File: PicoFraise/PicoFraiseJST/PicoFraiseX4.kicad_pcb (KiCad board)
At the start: 2 copper layers, 112.8 x 110 mm, 76 parts, among them J1 Conn_01x06, J2 Conn_01x06, J3 Conn_01x06, J4 Conn_01x06, J5 Conn_01x09, J7 Reset, J8 12-24V input, U1 Pico, U2 L7805

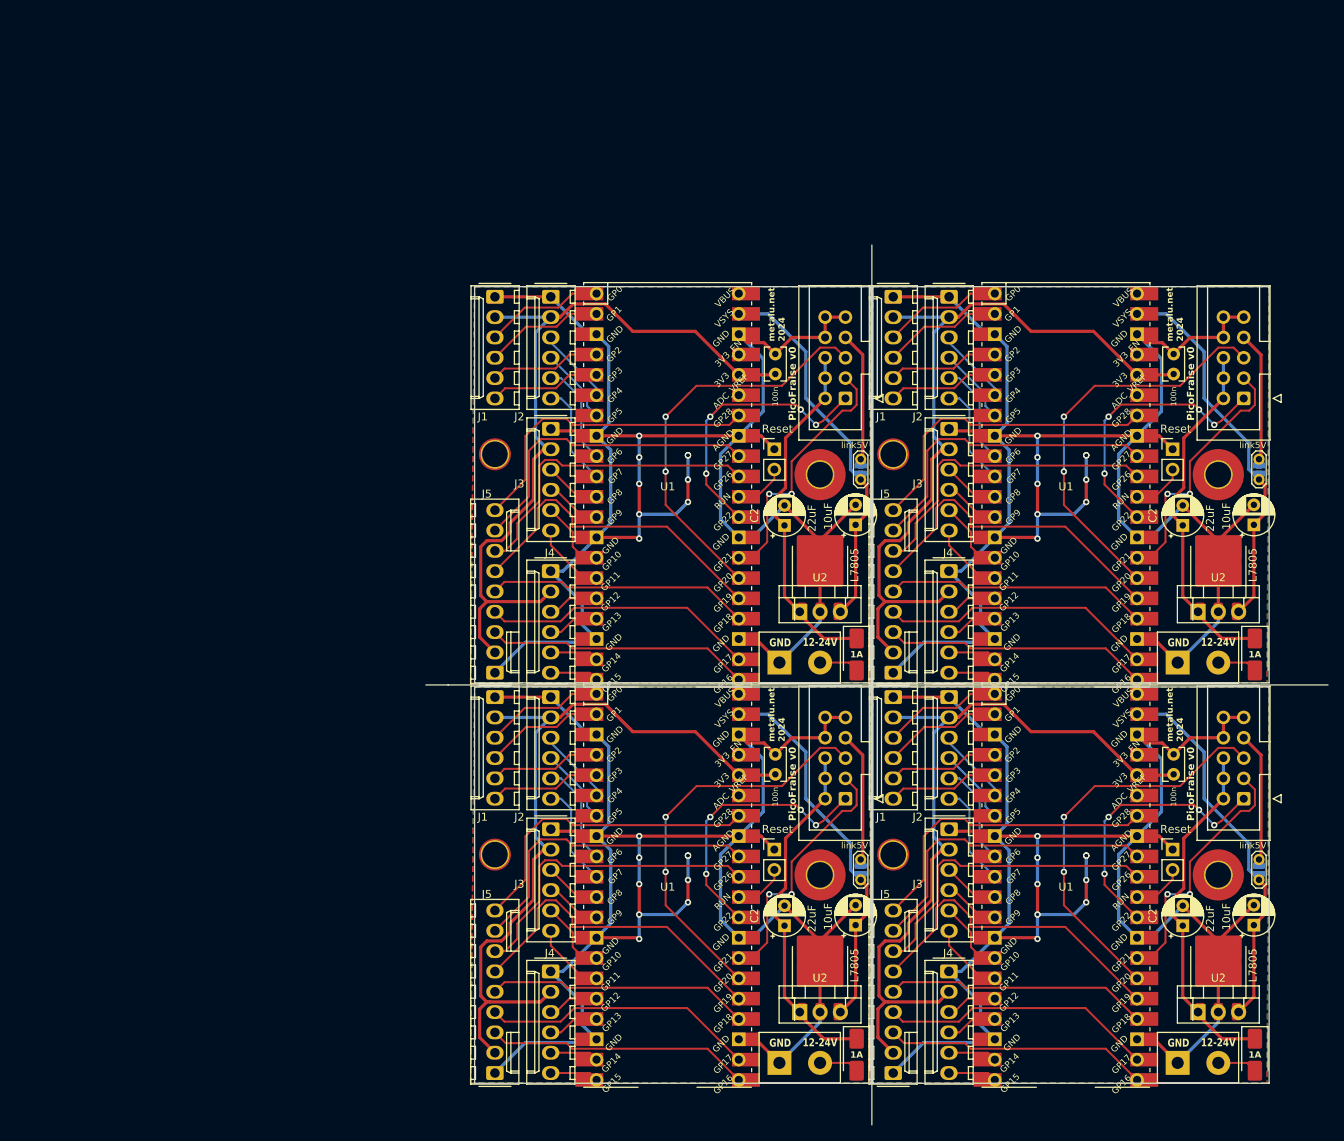
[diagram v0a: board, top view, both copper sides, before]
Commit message: update PicoFraiseJST
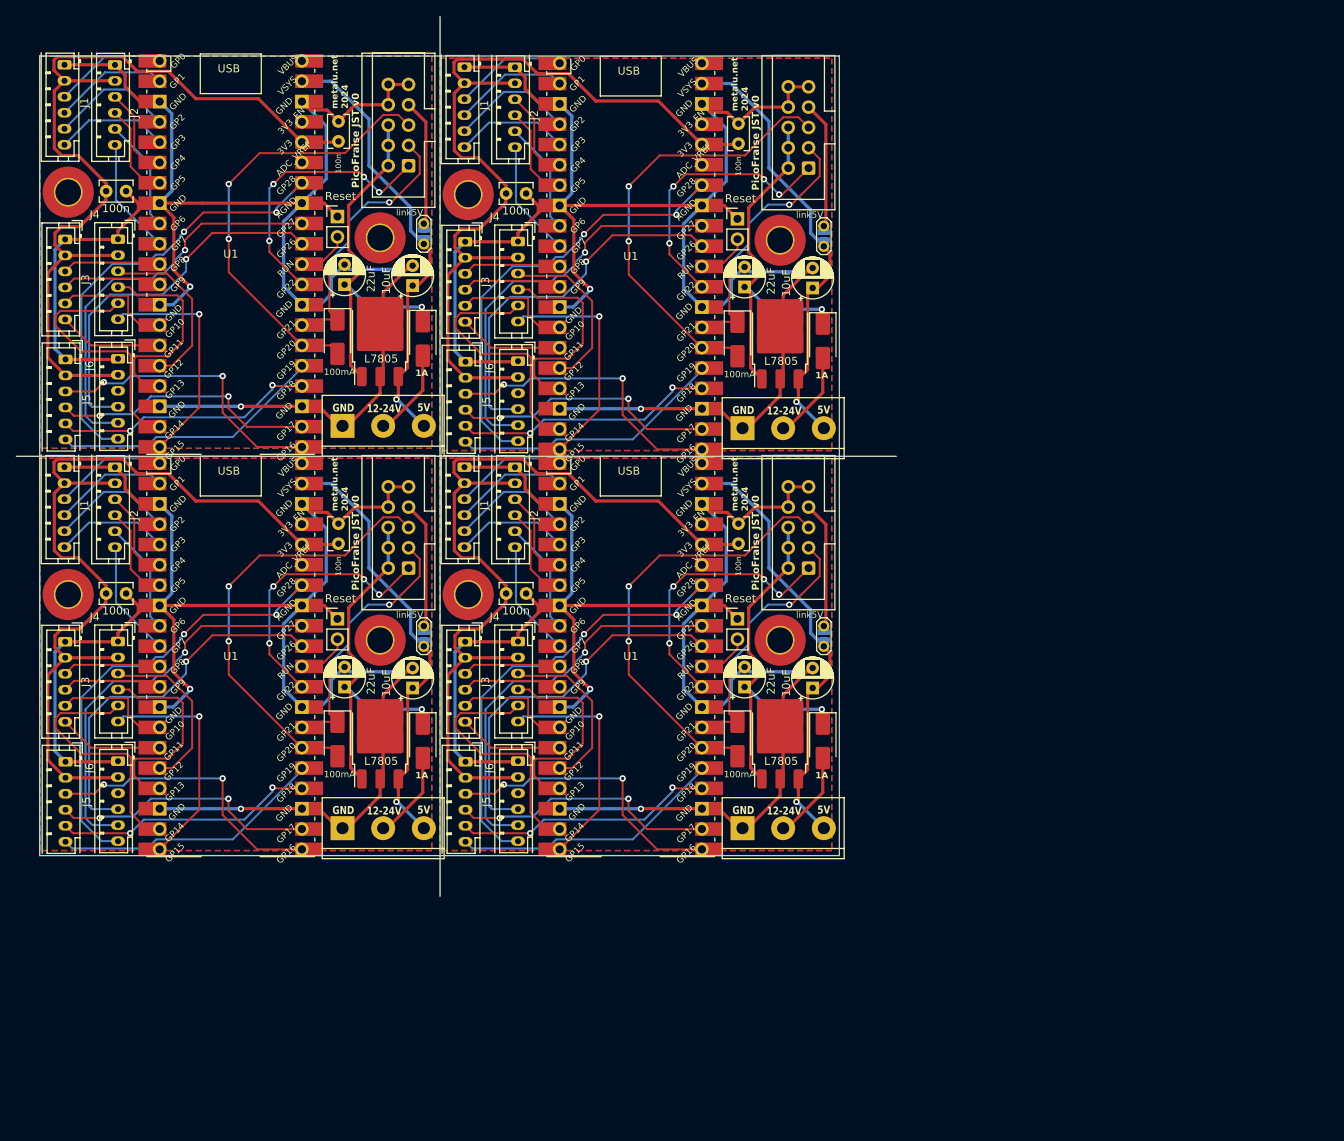
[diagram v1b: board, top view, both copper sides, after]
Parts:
- removed the C1 at (201.7, 124.5)
- removed the C1 at (201.7, 74.4)
- removed the C1 at (151.9, 74.4)
- removed the C1 at (151.9, 124.5)
- removed the C2 at (202.8, 93.3)
- removed the C2 at (202.8, 143.4)
- removed the C2 at (153.0, 93.3)
- removed the C2 at (153.0, 143.4)
- removed the C3 at (211.7, 93.3)
- removed the C3 at (161.9, 143.3)
- removed the C3 at (161.9, 93.3)
- removed the C3 at (211.7, 143.3)
- removed the D1 at (211.8, 109.5)
- removed the D1 at (162.1, 109.5)
- removed the D1 at (162.1, 159.5)
- removed the D1 at (211.8, 159.5)
- removed the FR1 at (160.7, 127.5)
- removed the FR1 at (210.4, 127.5)
- removed the FR1 at (210.4, 77.5)
- removed the FR1 at (160.7, 77.5)
- removed the H1 at (166.6, 84.5)
- removed the H1 at (116.8, 84.5)
- removed the H1 at (116.8, 134.5)
- removed the H1 at (166.6, 134.5)
- removed the H2 at (207.3, 87.0)
- removed the H2 at (207.3, 137.0)
- removed the H2 at (157.5, 137.0)
- removed the H2 at (157.5, 87.0)
- removed the J1 at (116.8, 64.8)
- removed the J1 at (166.6, 64.8)
- removed the J1 at (166.6, 114.8)
- removed the J1 at (116.8, 114.8)
- removed the J2 at (123.8, 64.8)
- removed the J2 at (173.6, 114.8)
- removed the J2 at (123.8, 114.8)
- removed the J2 at (173.6, 64.8)
- removed the J3 at (123.8, 81.3)
- removed the J3 at (123.8, 131.3)
- removed the J3 at (173.6, 131.3)
- removed the J3 at (173.6, 81.3)
- removed the J4 at (123.8, 99.1)
- removed the J4 at (123.8, 149.1)
- removed the J4 at (173.6, 149.1)
- removed the J4 at (173.6, 99.1)
- removed the J5 at (116.8, 111.8)
- removed the J5 at (116.8, 161.8)
- removed the J5 at (166.6, 161.8)
- removed the J5 at (166.6, 111.8)
- removed the J7 at (201.5, 133.9)
- removed the J7 at (151.8, 83.8)
- removed the J7 at (201.5, 83.8)
- removed the J7 at (151.8, 133.9)
- removed the J8 at (152.4, 160.5)
- removed the J8 at (152.4, 110.5)
- removed the J8 at (202.2, 110.5)
- removed the J8 at (202.2, 160.5)
- removed the JP1 at (162.6, 86.4)
- removed the JP1 at (162.6, 136.4)
- removed the JP1 at (212.3, 136.4)
- removed the JP1 at (212.3, 86.4)
- removed the JP2 at (162.6, 137.6)
- removed the JP2 at (212.3, 87.6)
- removed the JP2 at (162.6, 87.6)
- removed the JP2 at (212.3, 137.6)
- removed the U1 at (188.2, 138.5)
- removed the U1 at (138.4, 138.5)
- removed the U1 at (138.4, 88.5)
- removed the U1 at (188.2, 88.5)
- removed U2 (x4): L7805, Package_TO_SOT_THT:TO-220-3_Vertical
- removed the Ubis2 at (157.5, 149.1)
- removed the Ubis2 at (157.5, 99.0)
- removed the Ubis2 at (207.3, 99.0)
- removed the Ubis2 at (207.3, 149.1)
- added C1: 100n, Capacitor_THT:C_Rect_L4.0mm_W2.5mm_P2.50mm, F.Cu at (147.3, 95.6)
- added C1: 100n, Capacitor_THT:C_Rect_L4.0mm_W2.5mm_P2.50mm, F.Cu at (97.3, 95.6)
- added C1: 100n, Capacitor_THT:C_Rect_L4.0mm_W2.5mm_P2.50mm, F.Cu at (147.3, 45.6)
- added C1: 100n, Capacitor_THT:C_Rect_L4.0mm_W2.5mm_P2.50mm, F.Cu at (97.3, 45.3)
- added C2: 22uF, Capacitor_THT:CP_Radial_D5.0mm_P2.50mm, F.Cu at (148.0, 63.5)
- added C2: 22uF, Capacitor_THT:CP_Radial_D5.0mm_P2.50mm, F.Cu at (148.0, 113.5)
- added C2: 22uF, Capacitor_THT:CP_Radial_D5.0mm_P2.50mm, F.Cu at (98.0, 113.5)
- added C2: 22uF, Capacitor_THT:CP_Radial_D5.0mm_P2.50mm, F.Cu at (98.0, 63.2)
- added C3: 10uF, Capacitor_THT:CP_Radial_D5.0mm_P2.50mm, F.Cu at (106.6, 113.7)
- added C3: 10uF, Capacitor_THT:CP_Radial_D5.0mm_P2.50mm, F.Cu at (156.6, 63.7)
- added C3: 10uF, Capacitor_THT:CP_Radial_D5.0mm_P2.50mm, F.Cu at (106.6, 63.4)
- added C3: 10uF, Capacitor_THT:CP_Radial_D5.0mm_P2.50mm, F.Cu at (156.6, 113.7)
- added C4: 100n, Capacitor_THT:C_Rect_L4.0mm_W2.5mm_P2.50mm, F.Cu at (118.2, 51.9)
- added C4: 100n, Capacitor_THT:C_Rect_L4.0mm_W2.5mm_P2.50mm, F.Cu at (68.2, 101.9)
- added C4: 100n, Capacitor_THT:C_Rect_L4.0mm_W2.5mm_P2.50mm, F.Cu at (118.2, 101.9)
- added C4: 100n, Capacitor_THT:C_Rect_L4.0mm_W2.5mm_P2.50mm, F.Cu at (68.2, 51.6)
- added D1: 1A, Diode_SMD:D_SMA, F.Cu at (157.8, 70.3)
- added D1: 1A, Diode_SMD:D_SMA, F.Cu at (107.8, 70.0)
- added D1: 1A, Diode_SMD:D_SMA, F.Cu at (157.8, 120.3)
- added D1: 1A, Diode_SMD:D_SMA, F.Cu at (107.8, 120.3)
- added D2: 100mA, Diode_SMD:D_SMA, F.Cu at (147.2, 120.0)
- added D2: 100mA, Diode_SMD:D_SMA, F.Cu at (97.2, 69.8)
- added D2: 100mA, Diode_SMD:D_SMA, F.Cu at (97.2, 120.0)
- added D2: 100mA, Diode_SMD:D_SMA, F.Cu at (147.2, 70.0)
- added FR1: Fraise_5x2, Connector_IDC:IDC-Header_2x05_P2.54mm_Vertical, F.Cu at (106.0, 98.7)
- added FR1: Fraise_5x2, Connector_IDC:IDC-Header_2x05_P2.54mm_Vertical, F.Cu at (156.0, 98.7)
- added FR1: Fraise_5x2, Connector_IDC:IDC-Header_2x05_P2.54mm_Vertical, F.Cu at (106.0, 48.4)
- added FR1: Fraise_5x2, Connector_IDC:IDC-Header_2x05_P2.54mm_Vertical, F.Cu at (156.0, 48.7)
- added H1: MountingHole, MountingHole:MountingHole_3.2mm_M3_Pad_TopOnly, F.Cu at (63.5, 51.7)
- added H1: MountingHole, MountingHole:MountingHole_3.2mm_M3_Pad_TopOnly, F.Cu at (63.5, 102.0)
- added H1: MountingHole, MountingHole:MountingHole_3.2mm_M3_Pad_TopOnly, F.Cu at (113.5, 102.0)
- added H1: MountingHole, MountingHole:MountingHole_3.2mm_M3_Pad_TopOnly, F.Cu at (113.5, 52.0)
- added H2: MountingHole, MountingHole:MountingHole_3.2mm_M3_Pad_TopOnly, F.Cu at (152.5, 107.7)
- added H2: MountingHole, MountingHole:MountingHole_3.2mm_M3_Pad_TopOnly, F.Cu at (102.5, 57.4)
- added H2: MountingHole, MountingHole:MountingHole_3.2mm_M3_Pad_TopOnly, F.Cu at (102.5, 107.7)
- added H2: MountingHole, MountingHole:MountingHole_3.2mm_M3_Pad_TopOnly, F.Cu at (152.5, 57.7)
- added J1: Conn_01x06, Connector_JST:JST_PH_B6B-PH-K_1x06_P2.00mm_Vertical, F.Cu at (63.0, 35.8)
- added J1: Conn_01x06, Connector_JST:JST_PH_B6B-PH-K_1x06_P2.00mm_Vertical, F.Cu at (113.0, 86.1)
- added J1: Conn_01x06, Connector_JST:JST_PH_B6B-PH-K_1x06_P2.00mm_Vertical, F.Cu at (113.0, 36.1)
- added J1: Conn_01x06, Connector_JST:JST_PH_B6B-PH-K_1x06_P2.00mm_Vertical, F.Cu at (63.0, 86.1)
- added J2: Conn_01x06, Connector_JST:JST_PH_B6B-PH-K_1x06_P2.00mm_Vertical, F.Cu at (69.3, 35.8)
- added J2: Conn_01x06, Connector_JST:JST_PH_B6B-PH-K_1x06_P2.00mm_Vertical, F.Cu at (119.3, 36.1)
- added J2: Conn_01x06, Connector_JST:JST_PH_B6B-PH-K_1x06_P2.00mm_Vertical, F.Cu at (69.3, 86.1)
- added J2: Conn_01x06, Connector_JST:JST_PH_B6B-PH-K_1x06_P2.00mm_Vertical, F.Cu at (119.3, 86.1)
- added J3: Conn_01x06, Connector_JST:JST_PH_B6B-PH-K_1x06_P2.00mm_Vertical, F.Cu at (113.1, 57.9)
- added J3: Conn_01x06, Connector_JST:JST_PH_B6B-PH-K_1x06_P2.00mm_Vertical, F.Cu at (113.1, 107.9)
- added J3: Conn_01x06, Connector_JST:JST_PH_B6B-PH-K_1x06_P2.00mm_Vertical, F.Cu at (63.1, 107.9)
- added J3: Conn_01x06, Connector_JST:JST_PH_B6B-PH-K_1x06_P2.00mm_Vertical, F.Cu at (63.1, 57.6)
- added J4: Conn_01x06, Connector_JST:JST_PH_B6B-PH-K_1x06_P2.00mm_Vertical, F.Cu at (119.7, 57.9)
- added J4: Conn_01x06, Connector_JST:JST_PH_B6B-PH-K_1x06_P2.00mm_Vertical, F.Cu at (69.7, 107.9)
- added J4: Conn_01x06, Connector_JST:JST_PH_B6B-PH-K_1x06_P2.00mm_Vertical, F.Cu at (119.7, 107.9)
- added J4: Conn_01x06, Connector_JST:JST_PH_B6B-PH-K_1x06_P2.00mm_Vertical, F.Cu at (69.7, 57.6)
- added J5: Conn_01x06, Connector_JST:JST_PH_B6B-PH-K_1x06_P2.00mm_Vertical, F.Cu at (63.2, 72.6)
- added J5: Conn_01x06, Connector_JST:JST_PH_B6B-PH-K_1x06_P2.00mm_Vertical, F.Cu at (113.2, 72.9)
- added J5: Conn_01x06, Connector_JST:JST_PH_B6B-PH-K_1x06_P2.00mm_Vertical, F.Cu at (113.2, 122.9)
- added J5: Conn_01x06, Connector_JST:JST_PH_B6B-PH-K_1x06_P2.00mm_Vertical, F.Cu at (63.2, 122.9)
- added J6: Conn_01x06, Connector_JST:JST_PH_B6B-PH-K_1x06_P2.00mm_Vertical, F.Cu at (69.7, 72.5)
- added J6: Conn_01x06, Connector_JST:JST_PH_B6B-PH-K_1x06_P2.00mm_Vertical, F.Cu at (119.7, 72.8)
- added J6: Conn_01x06, Connector_JST:JST_PH_B6B-PH-K_1x06_P2.00mm_Vertical, F.Cu at (69.7, 122.8)
- added J6: Conn_01x06, Connector_JST:JST_PH_B6B-PH-K_1x06_P2.00mm_Vertical, F.Cu at (119.7, 122.8)
- added J7: Reset, Connector_PinHeader_2.54mm:PinHeader_1x02_P2.54mm_Vertical, F.Cu at (97.2, 54.7)
- added J7: Reset, Connector_PinHeader_2.54mm:PinHeader_1x02_P2.54mm_Vertical, F.Cu at (147.2, 55.0)
- added J7: Reset, Connector_PinHeader_2.54mm:PinHeader_1x02_P2.54mm_Vertical, F.Cu at (97.2, 105.0)
- added J7: Reset, Connector_PinHeader_2.54mm:PinHeader_1x02_P2.54mm_Vertical, F.Cu at (147.2, 105.0)
- added J8: 12-24V input, TerminalBlock:TerminalBlock_bornier-3_P5.08mm, F.Cu at (147.8, 81.2)
- added J8: 12-24V input, TerminalBlock:TerminalBlock_bornier-3_P5.08mm, F.Cu at (97.8, 131.2)
- added J8: 12-24V input, TerminalBlock:TerminalBlock_bornier-3_P5.08mm, F.Cu at (147.8, 131.2)
- added J8: 12-24V input, TerminalBlock:TerminalBlock_bornier-3_P5.08mm, F.Cu at (97.8, 80.9)
- added JP1: link5V, Jumper:SolderJumper-2_P1.3mm_Open_RoundedPad1.0x1.5mm, B.Cu at (157.9, 57.2)
- added JP1: link5V, Jumper:SolderJumper-2_P1.3mm_Open_RoundedPad1.0x1.5mm, B.Cu at (108.0, 107.2)
- added JP1: link5V, Jumper:SolderJumper-2_P1.3mm_Open_RoundedPad1.0x1.5mm, B.Cu at (157.9, 107.2)
- added JP1: link5V, Jumper:SolderJumper-2_P1.3mm_Open_RoundedPad1.0x1.5mm, B.Cu at (108.0, 56.9)
- added JP2: link5V, TestPoint:TestPoint_2Pads_Pitch2.54mm_Drill0.8mm, F.Cu at (157.9, 58.5)
- added JP2: link5V, TestPoint:TestPoint_2Pads_Pitch2.54mm_Drill0.8mm, F.Cu at (108.0, 108.5)
- added JP2: link5V, TestPoint:TestPoint_2Pads_Pitch2.54mm_Drill0.8mm, F.Cu at (157.9, 108.5)
- added JP2: link5V, TestPoint:TestPoint_2Pads_Pitch2.54mm_Drill0.8mm, F.Cu at (108.0, 58.2)
- added U1: Pico, MCU_RaspberryPi_and_Boards:RPi_Pico_SMD_TH, F.Cu at (83.8, 59.4)
- added U1: Pico, MCU_RaspberryPi_and_Boards:RPi_Pico_SMD_TH, F.Cu at (133.8, 109.7)
- added U1: Pico, MCU_RaspberryPi_and_Boards:RPi_Pico_SMD_TH, F.Cu at (133.8, 59.7)
- added U1: Pico, MCU_RaspberryPi_and_Boards:RPi_Pico_SMD_TH, F.Cu at (83.8, 109.7)
- added Ubis2: L7805, Package_TO_SOT_SMD:TO-252-3_TabPin2, F.Cu at (102.5, 69.6)
- added Ubis2: L7805, Package_TO_SOT_SMD:TO-252-3_TabPin2, F.Cu at (152.5, 119.9)
- added Ubis2: L7805, Package_TO_SOT_SMD:TO-252-3_TabPin2, F.Cu at (102.5, 119.9)
- added Ubis2: L7805, Package_TO_SOT_SMD:TO-252-3_TabPin2, F.Cu at (152.5, 69.9)
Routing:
- net Net-(J6-Pin_6): track 0.00 -> 226.2 mm, vias 0 -> 8
- net Net-(J6-Pin_5): track 0.00 -> 201.1 mm, vias 0 -> 4
- net Net-(J6-Pin_4): track 0.00 -> 188.6 mm, vias 0 -> 4
- net Net-(J5-Pin_7): track 159.0 -> 0.00 mm
- net Net-(J5-Pin_8): track 157.8 -> 0.00 mm
- net Net-(J5-Pin_9): track 156.9 -> 0.00 mm
- net Net-(J4-Pin_5): track 24.4 -> 128.0 mm
- net Net-(J4-Pin_6): track 24.4 -> 116.3 mm, vias 0 -> 4
- net Net-(J4-Pin_4): track 25.7 -> 106.2 mm
- net Net-(J4-Pin_3): track 25.7 -> 86.6 mm
- net +3.3V: track 393.5 -> 441.9 mm
- net +5V: track 189.5 -> 225.2 mm, vias 0 -> 4
- net Net-(J3-Pin_3): track 28.5 -> 58.6 mm
- net Net-(J5-Pin_6): track 166.0 -> 136.9 mm
- net Net-(J3-Pin_4): track 28.5 -> 57.0 mm
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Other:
- board size 112.8 x 110 mm -> 110 x 110 mm
- board text added: "J6"
- board text added: "PicoFraise JST v0"
- board text added: "USB"
- board text added: "locked"
- board text removed: "PicoFraise v0"
- board text removed: "V-CUT"
